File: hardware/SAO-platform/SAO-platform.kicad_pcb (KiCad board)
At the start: 2 copper layers, 37 x 35 mm, 60 parts, among them U1 WCH CH32V003F4U6

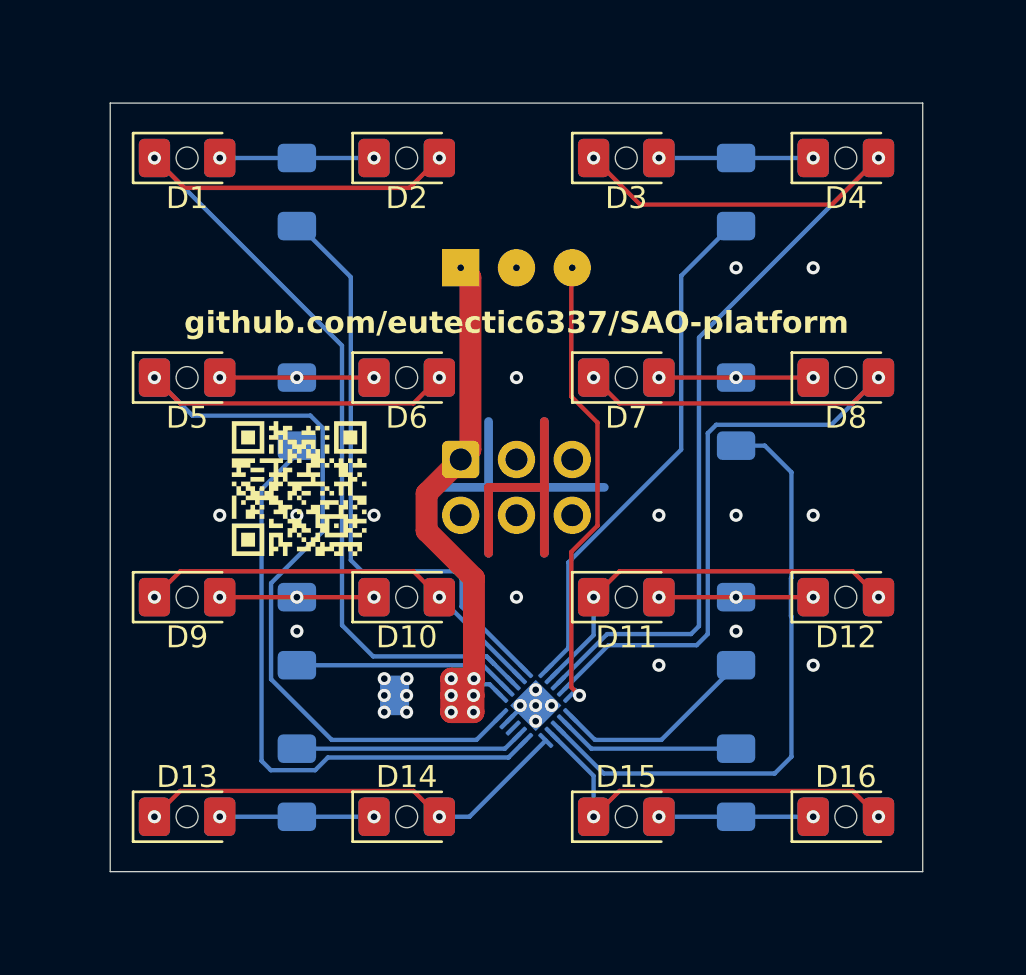
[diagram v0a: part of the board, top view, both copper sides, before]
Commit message: shrink the board
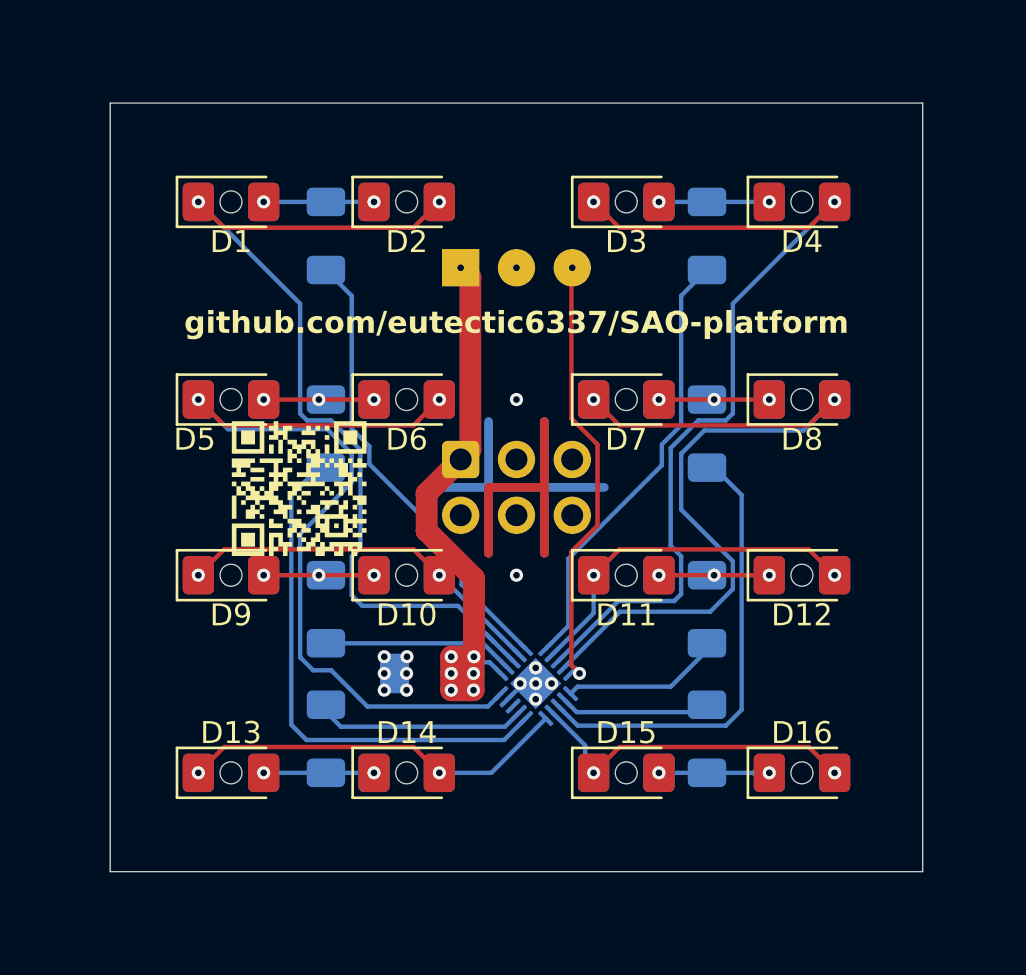
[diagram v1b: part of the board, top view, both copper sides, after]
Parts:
- moved D1 2.83 mm to (87.0, 87.0)
- moved D13 2.83 mm to (87.0, 113.0)
- moved D16 2.83 mm to (113.0, 113.0)
- moved D4 2.83 mm to (113.0, 87.0)
- moved h10 2.83 mm to (87.0, 87.0)
- moved h13 2.83 mm to (87.0, 113.0)
- moved h14 2.83 mm to (113.0, 113.0)
- moved h9 2.83 mm to (113.0, 87.0)
- moved rD1 2.83 mm to (87.0, 87.0)
- moved rD13 2.83 mm to (87.0, 113.0)
- moved rD16 2.83 mm to (113.0, 113.0)
- moved rD4 2.83 mm to (113.0, 87.0)
- moved R1 2.40 mm to (91.3, 88.6)
- moved R2 2.40 mm to (108.7, 88.6)
- moved R7 2.40 mm to (91.3, 111.4)
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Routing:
- net PWM4: track 27.8 -> 20.9 mm
- net GP3: track 47.0 -> 40.5 mm
- net GP2: track 46.9 -> 40.7 mm
- net PWM1: track 27.1 -> 21.0 mm
- net GP1: track 48.3 -> 42.8 mm
- net PWM3: track 27.8 -> 23.6 mm
- net PWM2: track 24.0 -> 20.3 mm
- net GP4: track 39.5 -> 36.2 mm
- net GP8: track 18.5 -> 15.5 mm
- net GP7: track 20.2 -> 17.8 mm
- net Net-(D7-A): track 7.03 -> 5.03 mm
- net Net-(D5-A): track 7.03 -> 5.03 mm
- net Net-(D3-A): track 7.03 -> 5.03 mm
- net Net-(D13-A): track 7.03 -> 5.03 mm
- net Net-(D11-A): track 7.85 -> 5.85 mm
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
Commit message: shrunk to 8mm grid for LED centres
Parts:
- moved PROG1 2.00 mm to (97.5, 92.0)
- moved D1 1.41 mm to (88.0, 88.0)
- moved D13 1.41 mm to (88.0, 112.0)
- moved D14 1.41 mm to (96.0, 112.0)
- moved D15 1.41 mm to (104.0, 112.0)
- moved D16 1.41 mm to (112.0, 112.0)
- moved D2 1.41 mm to (96.0, 88.0)
- moved D3 1.41 mm to (104.0, 88.0)
- moved D4 1.41 mm to (112.0, 88.0)
- moved h1 1.41 mm to (104.0, 88.0)
- moved h10 1.41 mm to (88.0, 88.0)
- moved h13 1.41 mm to (88.0, 112.0)
- moved h14 1.41 mm to (112.0, 112.0)
- moved h2 1.41 mm to (96.0, 88.0)
- moved h5 1.41 mm to (96.0, 112.0)
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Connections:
- U1 pad 1: PWM3 -> PWM7
- U1 pad 17: PWM8 -> PWM4
- U1 pad 18: PWM4 -> PWM8
- U1 pad 2: PWM7 -> PWM5
- U1 pad 7: PWM5 -> PWM3
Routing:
- net GND: track 1.62 -> 36.7 mm, vias 13 -> 12
- net +3V0: track 27.1 -> 18.0 mm
- net PWM3: track 23.6 -> 14.5 mm
- net GP3: track 40.5 -> 35.4 mm
- net GP4: track 36.2 -> 32.3 mm
- net GP1: track 42.8 -> 39.3 mm
- net GP2: track 40.7 -> 37.6 mm
- net PWM4: track 20.9 -> 17.8 mm
- net PWM5: track 9.02 -> 11.1 mm
- net /SWIO: track 19.6 -> 17.8 mm
- net GP7: track 17.8 -> 16.4 mm
- net GP8: track 15.5 -> 14.1 mm
- net Net-(D15-A): track 6.10 -> 5.03 mm
- net PWM6: track 7.48 -> 6.63 mm
- net Net-(D11-A): track 5.85 -> 5.03 mm
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- added copper zone on F.Cu, net +3V0
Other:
- board size 37 x 35 mm -> 31 x 31 mm
